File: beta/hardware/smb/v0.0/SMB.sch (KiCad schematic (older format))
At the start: 21 parts, among them IC101 ATMEGA1284-A, J101 I2C, J102 RTS_RESET, J103 ICSP, J104 SERIAL_REV, SW101 reset_sw, X101 16MHz

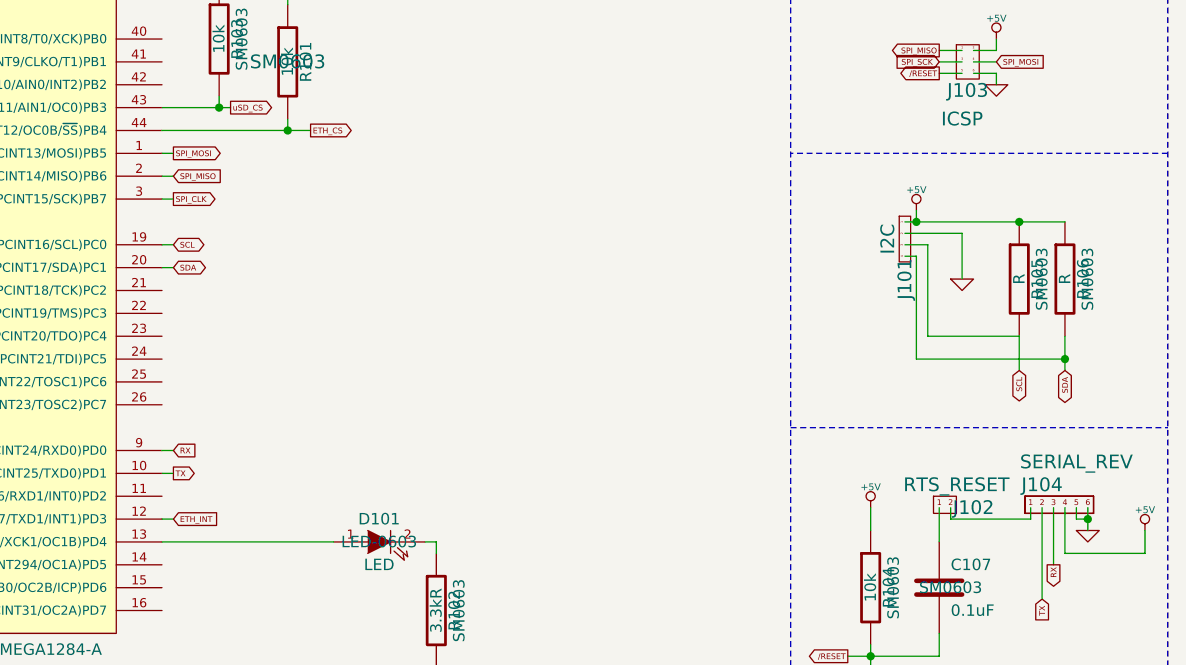
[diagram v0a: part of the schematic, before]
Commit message: Begining of the routing
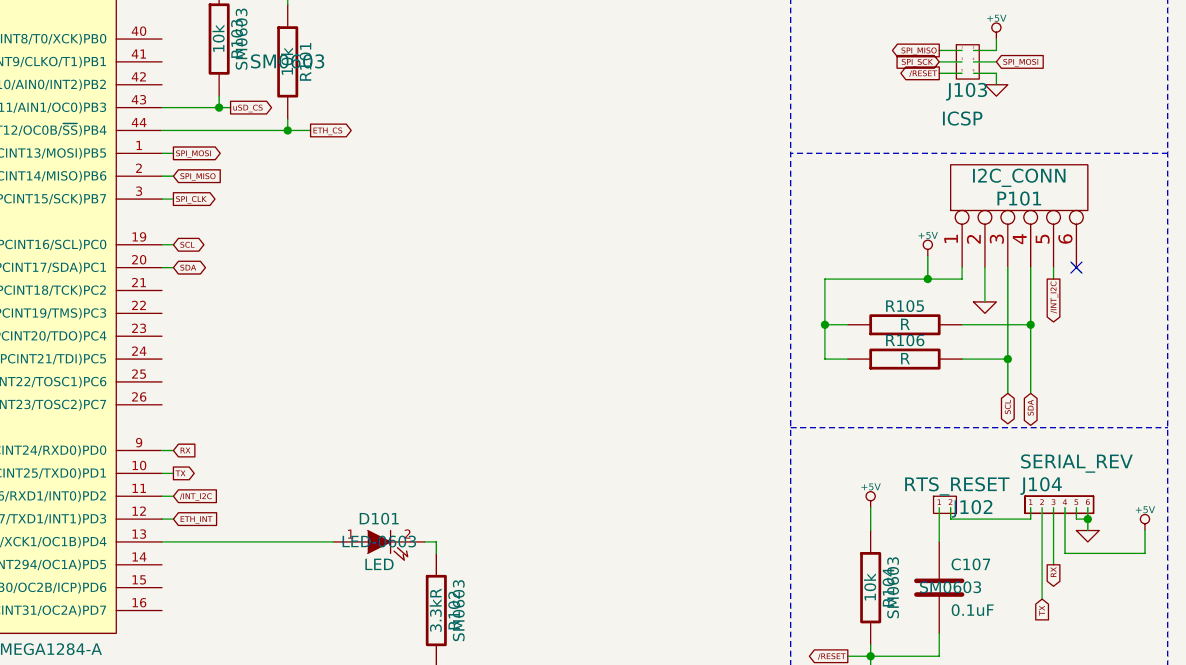
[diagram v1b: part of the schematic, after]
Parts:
- removed J101: I2C, symbol 4PIN
- added P101: I2C_CONN, symbol CONN_6
- R105, R106: footprint SM0603 -> (none)
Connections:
- net +5V: now also P101.1
- net GND: now also P101.2
- net SCL: now also R106.2, P101.3; no longer R105.2
- net SDA: now also R105.2, P101.4; no longer R106.2
- net /INT_I2C: now reaches IC101.11 ((PCINT26/RXD1/INT0)PD2)
- net /INT_I2C: now also P101.5
- no-connect marks 0 -> 1
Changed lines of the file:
@@
-EESchema Schematic File Version 2  date 15/07/2012 20:25:53
+EESchema Schematic File Version 2  date 23/07/2012 00:31:40
 LIBS:power
 LIBS:device
@@
 Sheet 1 4
 Title ""
-Date "15 jul 2012"
+Date "22 jul 2012"
 Rev ""
 Comp ""
@@
 $EndDescr
 Wire Wire Line
+	10450 4000 10450 4050
+Connection ~ 9450 4250
+Connection ~ 9900 4050
+Wire Wire Line
+	9450 4050 10050 4050
+Wire Wire Line
+	9450 4050 9450 4400
+Connection ~ 10250 4400
+Wire Wire Line
+	10050 4400 10250 4400
+Wire Wire Line
+	10250 4550 10250 4000
+Wire Wire Line
+	10150 4000 10150 4150
+Wire Wire Line
 	6800 2700 6800 2750
 Wire Wire Line
@@
 Wire Wire Line
 	6600 3900 6550 3900
-Wire Wire Line
-	10300 4450 10300 4300
-Wire Wire Line
-	10050 4050 10050 3850
-Wire Wire Line
-	10050 3850 9800 3850
-Wire Wire Line
-	10300 4300 9900 4300
-Wire Wire Line
-	9900 4300 9900 3900
-Wire Wire Line
-	9900 3900 9800 3900
-Connection ~ 9850 3800
 Wire Notes Line
 	9300 6150 10950 6150
@@
 	7100 2800 7100 2850
 Wire Wire Line
-	9850 3800 9850 3750
-Wire Wire Line
-	10500 3800 9800 3800
-Connection ~ 10300 3800
-Wire Wire Line
-	9800 3950 9850 3950
-Wire Wire Line
-	9850 3950 9850 4400
-Wire Wire Line
-	9850 4400 10500 4400
-Wire Wire Line
-	10500 4450 10500 4300
-Connection ~ 10500 4400
-Wire Wire Line
 	6600 4000 6550 4000
 Wire Notes Line
@@
 	6800 3250 6800 3300
 Connection ~ 6800 3300
+Wire Wire Line
+	9900 4050 9900 3950
+Wire Wire Line
+	10050 4050 10050 4000
+Wire Wire Line
+	10050 4250 10350 4250
+Connection ~ 10350 4250
+Wire Wire Line
+	10350 4550 10350 4000
+Wire Wire Line
+	9450 4400 9550 4400
+Wire Wire Line
+	9450 4250 9550 4250
+Wire Wire Line
+	6600 5000 6550 5000
+Text GLabel 10450 4050 3    25   Output ~ 0
+/INT_I2C
+Text GLabel 6600 5000 2    25   Input ~ 0
+/INT_I2C
+$Comp
+L R R105
+U 1 1 500C6C4F
+P 9800 4250
+F 0 "R105" V 9880 4250 50  0000 C CNN
+F 1 "R" V 9800 4250 50  0000 C CNN
+	1    9800 4250
+	0    -1   -1   0
+$EndComp
+$Comp
+L R R106
+U 1 1 500C6C3A
+P 9800 4400
+F 0 "R106" V 9880 4400 50  0000 C CNN
+F 1 "R" V 9800 4400 50  0000 C CNN
+	1    9800 4400
+	0    -1   -1   0
+$EndComp
+NoConn ~ 10550 4000
 $Comp
 L +5V #PWR01
+U 1 1 500C6B5D
+P 9900 3950
+F 0 "#PWR01" H 9900 4040 20  0001 C CNN
+F 1 "+5V" H 9900 4040 30  0000 C CNN
+	1    9900 3950
+	1    0    0    -1
+$EndComp
+$Comp
+L GND #PWR02
+U 1 1 500C6B4D
+P 10150 4150
+F 0 "#PWR02" H 10150 4150 30  0001 C CNN
+F 1 "GND" H 10150 4080 30  0001 C CNN
+	1    10150 4150
+	1    0    0    -1
+$EndComp
+$Comp
+L CONN_6 P101
+U 1 1 500C6B20
+P 10300 3650
+F 0 "P101" V 10250 3650 60  0000 C CNN
+F 1 "I2C_CONN" V 10350 3650 60  0000 C CNN
+	1    10300 3650
+	0    -1   -1   0
+$EndComp
+$Comp
+L +5V #PWR03
 U 1 1 4FF09080
 P 6800 2700
-F 0 "#PWR01" H 6800 2790 20  0001 C CNN
+F 0 "#PWR03" H 6800 2790 20  0001 C CNN
 F 1 "+5V" H 6800 2790 30  0000 C CNN
 	1    6800 2700
@@
 SPI_MOSI
 $Comp
-L +5V #PWR02
+L +5V #PWR04
 U 1 1 4FDE4559
 P 10200 3000
-F 0 "#PWR02" H 10200 3090 20  0001 C CNN
+F 0 "#PWR04" H 10200 3090 20  0001 C CNN
 F 1 "+5V" H 10200 3090 30  0000 C CNN
 	1    10200 3000
@@
 $EndComp
 $Comp
-L GND #PWR03
+L GND #PWR05
 U 1 1 4FDE454D
 P 10200 3200
-F 0 "#PWR03" H 10200 3200 30  0001 C CNN
+F 0 "#PWR05" H 10200 3200 30  0001 C CNN
 F 1 "GND" H 10200 3130 30  0001 C CNN
 	1    10200 3200
@@
 $EndSheet
 $Comp
-L +5V #PWR04
-U 1 1 4FDE1B12
-P 9850 3750
-F 0 "#PWR04" H 9850 3840 20  0001 C CNN
-F 1 "+5V" H 9850 3840 30  0000 C CNN
-	1    9850 3750
-	1    0    0    -1
-$EndComp
-$Comp
-L +5V #PWR05
+L +5V #PWR06
 U 1 1 4FDE1B05
 P 9650 5050
-F 0 "#PWR05" H 9650 5140 20  0001 C CNN
+F 0 "#PWR06" H 9650 5140 20  0001 C CNN
 F 1 "+5V" H 9650 5140 30  0000 C CNN
 	1    9650 5050
@@
 $EndComp
 $Comp
-L +5V #PWR06
+L +5V #PWR07
 U 1 1 4FDE1B01
 P 10850 5150
-F 0 "#PWR06" H 10850 5240 20  0001 C CNN
+F 0 "#PWR07" H 10850 5240 20  0001 C CNN
 F 1 "+5V" H 10850 5240 30  0000 C CNN
 	1    10850 5150
@@
 $EndComp
 $Comp
-L +5V #PWR07
+L +5V #PWR08
 U 1 1 4FDE1AEF
 P 7100 2800
-F 0 "#PWR07" H 7100 2890 20  0001 C CNN
+F 0 "#PWR08" H 7100 2890 20  0001 C CNN
 F 1 "+5V" H 7100 2890 30  0000 C CNN
 	1    7100 2800
@@
 $EndComp
 $Comp
-L +5V #PWR08
+L +5V #PWR09
 U 1 1 4FDE1AE0
 P 5350 1000
-F 0 "#PWR08" H 5350 1090 20  0001 C CNN
+F 0 "#PWR09" H 5350 1090 20  0001 C CNN
 F 1 "+5V" H 5350 1090 30  0000 C CNN
 	1    5350 1000
@@
 $EndComp
 $Comp
-L GND #PWR09
+L GND #PWR010
 U 1 1 4FDE0BAB
 P 5350 5900
-F 0 "#PWR09" H 5350 5900 30  0001 C CNN
+F 0 "#PWR010" H 5350 5900 30  0001 C CNN
 F 1 "GND" H 5350 5830 30  0001 C CNN
 	1    5350 5900
@@
 $EndComp
 $Comp
-L GND #PWR010
+L GND #PWR011
 U 1 1 4FDE0BA8
 P 5250 5900
-F 0 "#PWR010" H 5250 5900 30  0001 C CNN
+F 0 "#PWR011" H 5250 5900 30  0001 C CNN
 F 1 "GND" H 5250 5830 30  0001 C CNN
 	1    5250 5900
@@
 $EndComp
 $Comp
-L GND #PWR011
+L GND #PWR012
 U 1 1 4FDE0BA5
 P 5450 5900
-F 0 "#PWR011" H 5450 5900 30  0001 C CNN
+F 0 "#PWR012" H 5450 5900 30  0001 C CNN
 F 1 "GND" H 5450 5830 30  0001 C CNN
 	1    5450 5900
@@
 $EndComp
 $Comp
-L GND #PWR012
+L GND #PWR013
 U 1 1 4FDE0BA2
 P 5550 5900
-F 0 "#PWR012" H 5550 5900 30  0001 C CNN
+F 0 "#PWR013" H 5550 5900 30  0001 C CNN
 F 1 "GND" H 5550 5830 30  0001 C CNN
 	1    5550 5900
@@
 $EndComp
 $Comp
-L GND #PWR013
+L GND #PWR014
 U 1 1 4FDE09A7
 P 4850 1700
-F 0 "#PWR013" H 4850 1700 30  0001 C CNN
+F 0 "#PWR014" H 4850 1700 30  0001 C CNN
 F 1 "GND" H 4850 1630 30  0001 C CNN
 	1    4850 1700
@@
 $EndComp
 $Comp
-L GND #PWR014
+L GND #PWR015
 U 1 1 4FDE09A4
 P 4600 1700
-F 0 "#PWR014" H 4600 1700 30  0001 C CNN
+F 0 "#PWR015" H 4600 1700 30  0001 C CNN
 F 1 "GND" H 4600 1630 30  0001 C CNN
 	1    4600 1700
@@
 $EndComp
 $Comp
-L GND #PWR015
+L GND #PWR016
 U 1 1 4FDE09A1
 P 4350 1700
-F 0 "#PWR015" H 4350 1700 30  0001 C CNN
+F 0 "#PWR016" H 4350 1700 30  0001 C CNN
 F 1 "GND" H 4350 1630 30  0001 C CNN
 	1    4350 1700
@@
 $EndComp
 $Comp
-L GND #PWR016
+L GND #PWR017
 U 1 1 4FDE099C
 P 4100 1700
-F 0 "#PWR016" H 4100 1700 30  0001 C CNN
+F 0 "#PWR017" H 4100 1700 30  0001 C CNN
 F 1 "GND" H 4100 1630 30  0001 C CNN
 	1    4100 1700
@@
 Text GLabel 6600 4000 2    25   BiDi ~ 0
 SDA
-Text GLabel 10300 4450 3    25   BiDi ~ 0
+Text GLabel 10250 4550 3    25   BiDi ~ 0
 SCL
-Text GLabel 10500 4450 3    25   BiDi ~ 0
+Text GLabel 10350 4550 3    25   BiDi ~ 0
 SDA
 $Comp
-L GND #PWR017
-U 1 1 4FA06DB4
-P 10050 4050
-F 0 "#PWR017" H 10050 4050 30  0001 C CNN
-F 1 "GND" H 10050 3980 30  0001 C CNN
-	1    10050 4050
-	1    0    0    -1
-$EndComp
-$Comp
-L R R106
-U 1 1 4FA06D7A
-P 10500 4050
-F 0 "R106" V 10580 4050 50  0000 C CNN
-F 1 "R" V 10500 4050 50  0000 C CNN
-F 2 "SM0603" V 10600 4050 50  0000 C CNN
-	1    10500 4050
-	1    0    0    -1
-$EndComp
-$Comp
-L R R105
-U 1 1 4FA06D51
-P 10300 4050
-F 0 "R105" V 10380 4050 50  0000 C CNN
-F 1 "R" V 10300 4050 50  0000 C CNN
-F 2 "SM0603" V 10400 4050 50  0000 C CNN
-	1    10300 4050
-	1    0    0    -1
-$EndComp
-$Comp
-L 4PIN J101
-U 1 1 4FA06CC5
-P 9800 3850
-F 0 "J101" H 10000 3850 60  0000 C CNN
-F 1 "I2C" H 9825 3775 60  0000 C CNN
-	1    9800 3850
-	0    1    1    0
-$EndComp
-$Comp
 L R R101
